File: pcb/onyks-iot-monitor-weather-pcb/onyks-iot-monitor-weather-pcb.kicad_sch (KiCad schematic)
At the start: 17 parts, among them SW1 BOOT, SW2 ENABLE, U1 ESP32-WROOM-32D, U2 SHT30-DIS

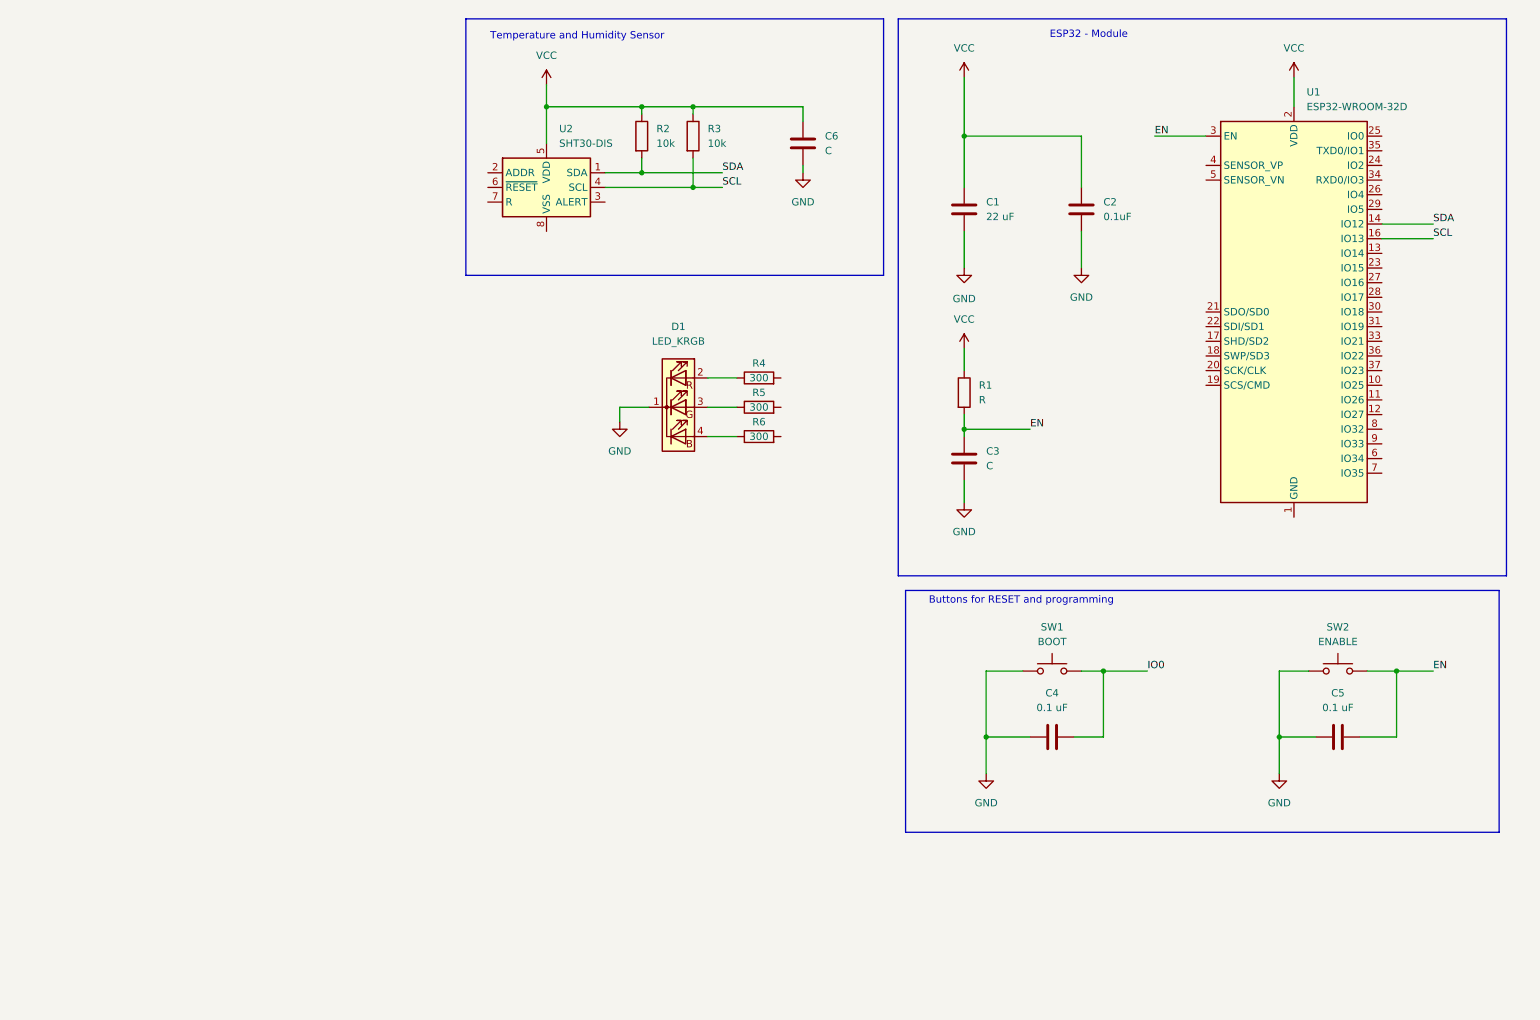
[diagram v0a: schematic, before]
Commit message: Added schematic for our project
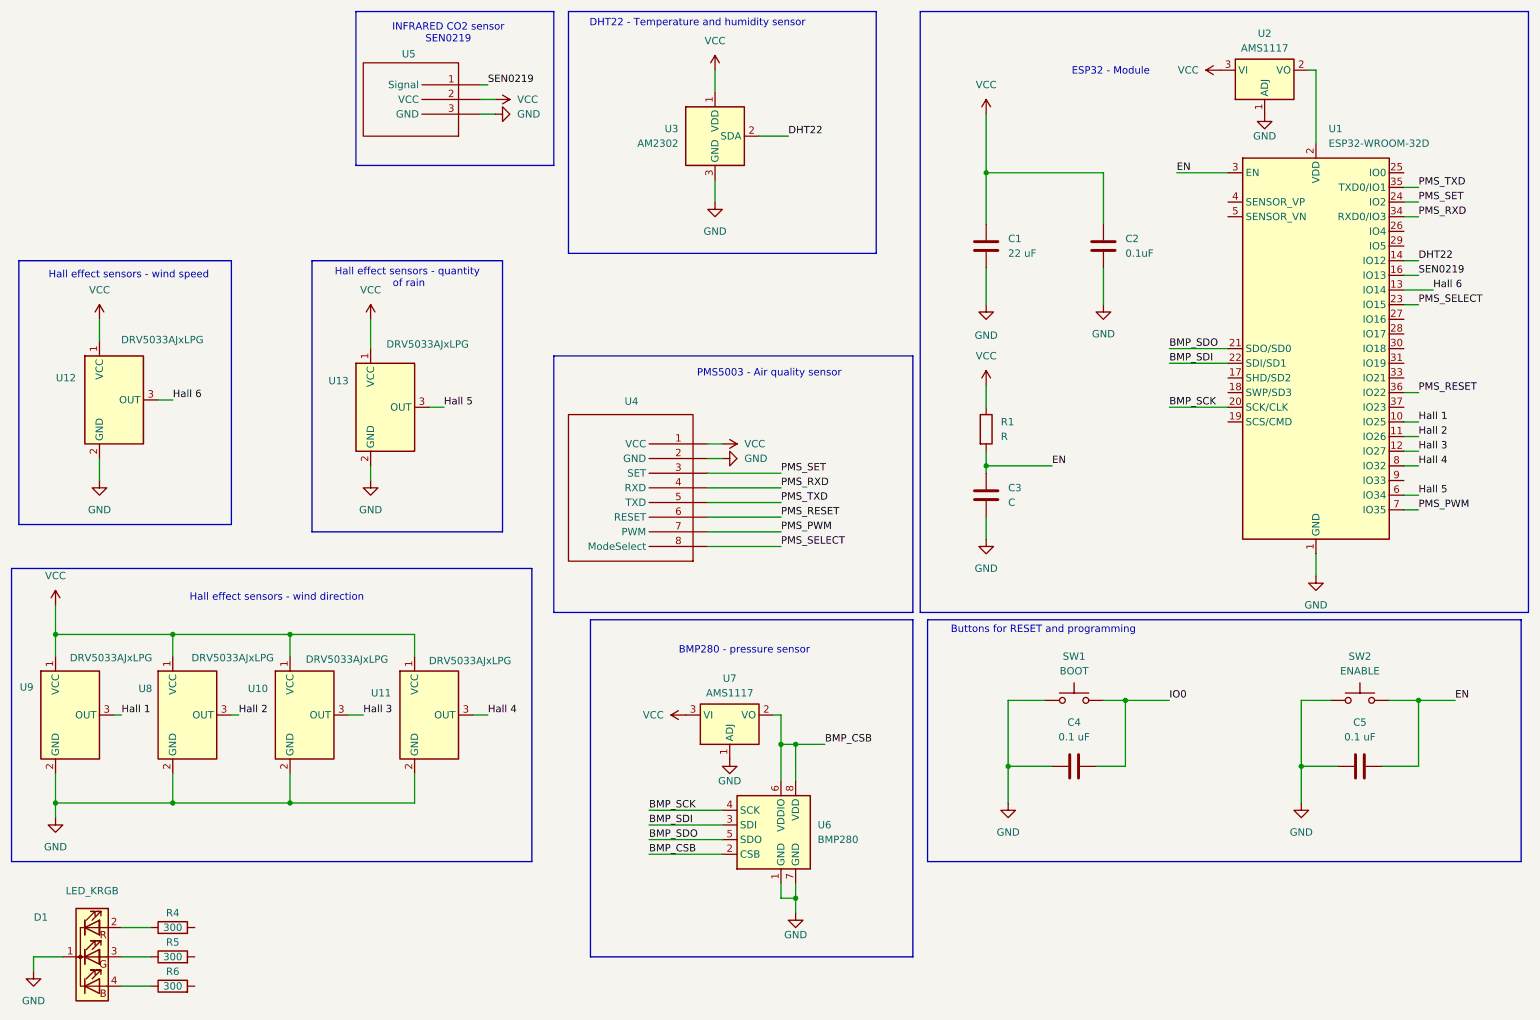
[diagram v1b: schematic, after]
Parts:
- removed C6: C, symbol Device:C
- removed R2, R3: 10k, symbol Device:R
- removed U2: SHT30-DIS, Sensor_Humidity:Sensirion_DFN-8-1EP_2.5x2.5mm_P0.5mm_EP1.1x1.7mm, symbol Sensor_Humidity:SHT30-DIS
- added U10, U11, U12, U13, U8, U9: DRV5033AJxLPG, Package_TO_SOT_THT:TO-92_Inline, symbol Sensor_Magnetic:DRV5033AJxLPG
- added U2, U7: AMS1117, Package_TO_SOT_SMD:SOT-223-3_TabPin2, symbol Regulator_Linear:AMS1117
- added U3: AM2302, Sensor:ASAIR_AM2302_P2.54mm_Vertical, symbol Sensor:AM2302
- added U4: ~, symbol 1BMoje:PMS5003
- added U5: ~, symbol 1BMoje:SEN0219
- added U6: BMP280, Package_LGA:Bosch_LGA-8_2x2.5mm_P0.65mm_ClockwisePinNumbering, symbol Sensor_Pressure:BMP280
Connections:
- net GND: now also U1.1 (GND), U1.15 (GND), U1.38 (GND), U1.39 (GND), U10.2 (GND), U11.2 (GND), U12.2 (GND), U13.2 (GND), U2.1 (ADJ), U3.3 (GND), U3.4 (GND), U4.2 (GND), U5.3 (GND), U6.1 (GND), U6.7 (GND), U7.1 (ADJ), U8.2 (GND), U9.2 (GND)
- net VCC: now also U10.1 (VCC), U11.1 (VCC), U12.1 (VCC), U13.1 (VCC), U2.3 (VI), U3.1 (VDD), U4.1 (VCC), U5.2 (VCC), U7.3 (VI), U8.1 (VCC), U9.1 (VCC); no longer U1.2 (VDD)
- net Hall 1: now reaches U1.10 (IO25)
- net Hall 1: now also U9.3 (OUT)
- net Hall 2: now reaches U1.11 (IO26)
- net Hall 2: now also U8.3 (OUT)
- net Hall 3: now reaches U1.12 (IO27)
- net Hall 3: now also U10.3 (OUT)
- net Hall 6: now reaches U1.13 (IO14)
- net Hall 6: now also U12.3 (OUT)
- net BMP_SCK: now reaches U1.20 (SCK/CLK)
- net BMP_SCK: now also U6.4 (SCK)
- net BMP_SDO: now reaches U1.21 (SDO/SD0)
- net BMP_SDO: now also U6.5 (SDO)
- net BMP_SDI: now reaches U1.22 (SDI/SD1)
- net BMP_SDI: now also U6.3 (SDI)
- net PMS_SELECT: now reaches U1.23 (IO15)
- net PMS_SELECT: now also U4.8 (ModeSelect)
- net PMS_SET: now reaches U1.24 (IO2)
- net PMS_SET: now also U4.3 (SET)
- net PMS_RXD: now reaches U1.34 (RXD0/IO3)
- net PMS_RXD: now also U4.4 (RXD)
- net PMS_TXD: now reaches U1.35 (TXD0/IO1)
- net PMS_TXD: now also U4.5 (TXD)
- net PMS_RESET: now reaches U1.36 (IO22)
- net PMS_RESET: now also U4.6 (RESET)
- net Hall 5: now reaches U1.6 (IO34)
- net Hall 5: now also U13.3 (OUT)
- net PMS_PWM: now reaches U1.7 (IO35)
- net PMS_PWM: now also U4.7 (PWM)
- net Hall 4: now reaches U1.8 (IO32)
- net Hall 4: now also U11.3 (OUT)
- net SCL renamed SEN0219
- net SEN0219: now also U5.1 (Signal)
- net SDA renamed DHT22
- net DHT22: now also U3.2 (SDA)
- new net: U1.2 (VDD), U2.2 (VO)
- new net BMP_CSB: U6.2 (CSB), U6.6 (VDDIO), U6.8 (VDD), U7.2 (VO)
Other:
- note added: "BMP280 - pressure sensor"
- note added: "DHT22 - Temperature and humidity sensor"
- note added: "Hall effect sensors - quantity of rain"
- note added: "Hall effect sensors - wind direction"
- note added: "Hall effect sensors - wind speed"
- note added: "INFRARED CO2 sensor SEN0219"
- note added: "PMS5003 - Air quality sensor"
- note removed: "Temperature and Humidity Sensor"
- moved on the sheet: C1, C2, C3, C4, C5, D1, R1, R4, R5, R6, SW1, SW2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
